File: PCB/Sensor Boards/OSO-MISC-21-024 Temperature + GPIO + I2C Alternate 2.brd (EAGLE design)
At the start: 14.4 x 7 mm, 8 parts, among them U2 LIS2DW12TR

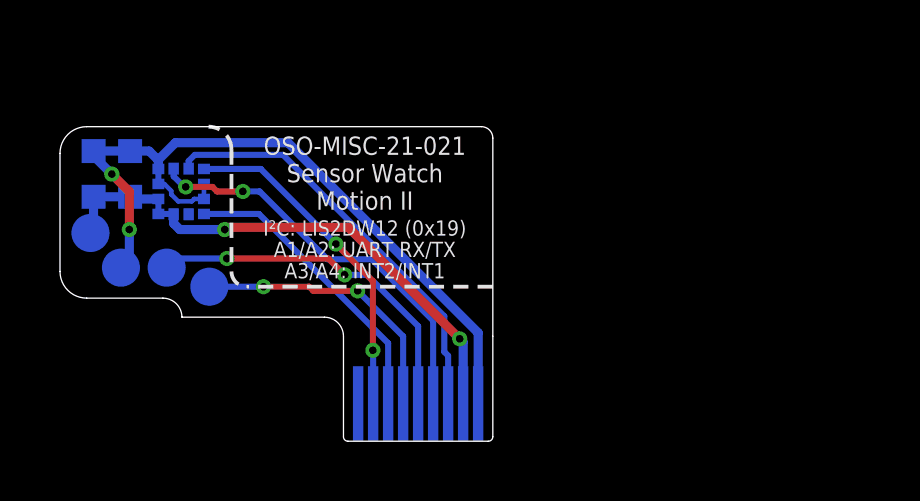
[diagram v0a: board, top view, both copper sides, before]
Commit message: more accelerometer and temperature board tests
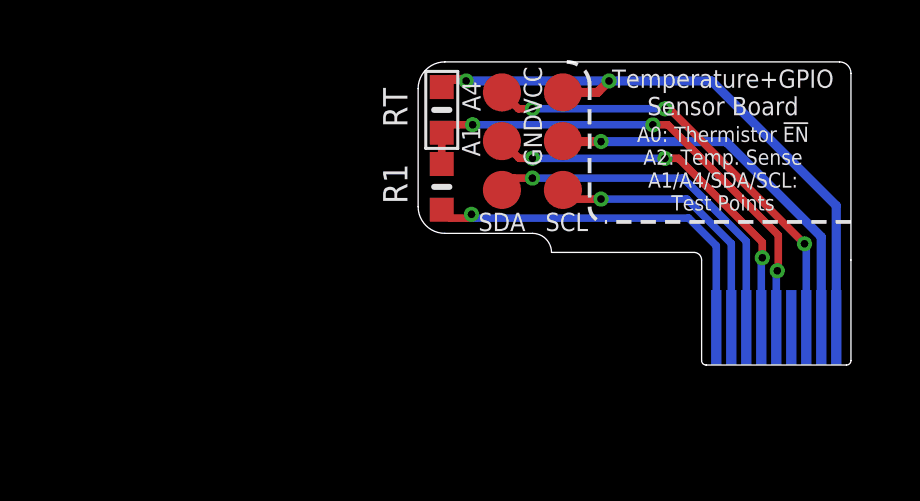
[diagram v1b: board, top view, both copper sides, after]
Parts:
- removed C1: 0.1uF, microbuilder:_0603MP
- removed C2: 10uF, microbuilder:_0603MP
- removed RX, TX, V+: TPB1,27, testpad:B1,27
- removed U2: LIS2DW12TR, LIS2DW12TR:LGA12R50P4X4_200X200X70
- added A1, A4, SCL, SDA, VCC: TPB1,27, testpad:B1,27
- added R1: 1% 10K, microbuilder:_0603MP
- added RT: NTC 10K, microbuilder:_0603MP
- moved GND 16.0 mm to (4.83, 3.71), flipped to the top
- moved U$3 12.2 mm to (11.9, -0.25)
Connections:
- removed net A0_UNUSED: U$3.9
- removed net A1_RX: RX.TP, U$3.6
- removed net A2_TX: TX.TP, U$3.5
- removed net A3_INT2: U$3.4, U2.11
- removed net A4_INT1: U$3.3, U2.12
- new net A0_TEMP_ENABLE: R1.2, U$3.9
- new net A1_SERCOM3.3: A1.TP, U$3.6
- new net A2_TEMP_SENSE: R1.1, RT.2, U$3.5
- new net A3: U$3.4
- new net A4_SERCOM3.2_TC3.0: A4.TP, U$3.3
- net GND: no longer C1.2, C2.1, U2.6, U2.7, U2.8
- net SCL: now also SCL.TP; no longer U2.1
- net SDA: now also SDA.TP; no longer U2.4
- net VCC: now also RT.1, VCC.TP; no longer C1.1, C2.2, U2.10, U2.2, U2.3, U2.9, V+.TP
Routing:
- net A2_TEMP_SENSE: track 0.00 -> 17.0 mm, vias 0 -> 3
- net A4_SERCOM3.2_TC3.0: track 0.00 -> 15.0 mm, vias 0 -> 3
- net A4_INT1: track 14.1 -> 0.00 mm
- net A3_INT2: track 13.7 -> 0.00 mm, vias 2 -> 0
- net A1_SERCOM3.3: track 0.00 -> 12.9 mm, vias 0 -> 3
- net A0_TEMP_ENABLE: track 0.00 -> 12.5 mm, vias 0 -> 1
- net A2_TX: track 12.0 -> 0.00 mm, vias 2 -> 0
- net A1_RX: track 9.39 -> 0.00 mm, vias 2 -> 0
- net GND: track 18.2 -> 13.0 mm, vias 2 -> 1
- net VCC: track 25.8 -> 20.8 mm
- net SCL: track 11.3 -> 9.15 mm, vias 2 -> 1
- net SDA: track 9.94 -> 12.1 mm, vias 0 -> 1
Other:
- board size 14.4 x 7 mm -> 14.4 x 6.6 mm
- board text added: "A0: Thermistor !EN A2: Temp. Sense A1/A4/SDA/SCL: Test Points"
- board text added: "A1/A4 Uses"
- board text added: "Digital IO Analog input PWM on TC3 UART RX/TX Interrupt 1/0 A4 ONLY: Ext. wake 0"
- board text added: "Temperature+GPIO Sensor Board"
- board text removed: "I²C: LIS2DW12 (0x19) A1/A2: UART RX/TX A3/A4: INT2/INT1"
- board text removed: "OSO-MISC-21-021 Sensor Watch Motion II"
